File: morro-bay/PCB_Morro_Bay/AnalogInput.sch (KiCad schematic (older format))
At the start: 95 parts, among them SW1 SW_DIP_x10, SW2 SW_DIP_x10, U10 LM2902, U11 LM2902, U12 LM2902, U5 LM2902, U6 LM2902, U7 LM2902, U8 LM2902, U9 LM2902

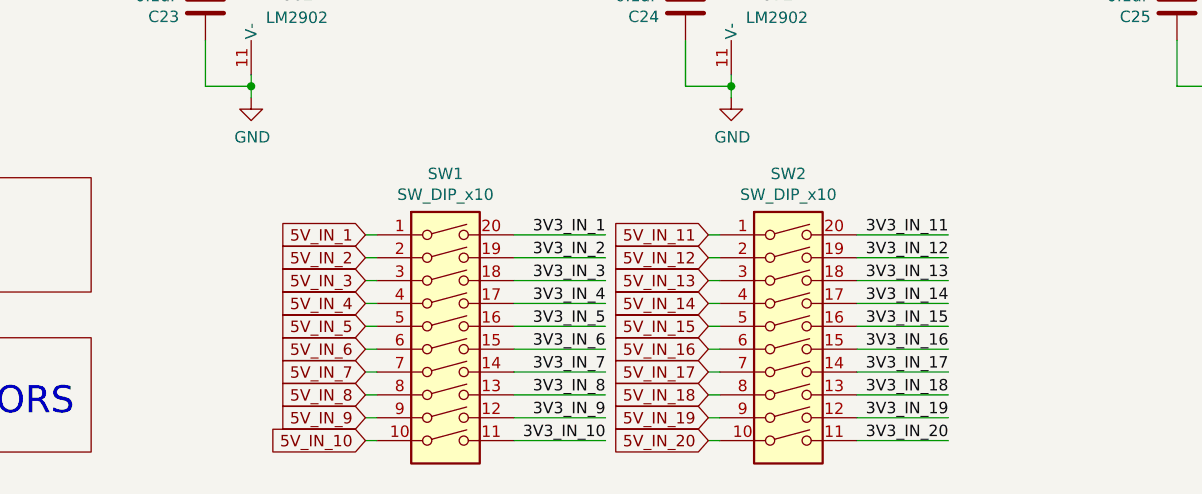
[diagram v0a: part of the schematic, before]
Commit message: Ready for initial sch review
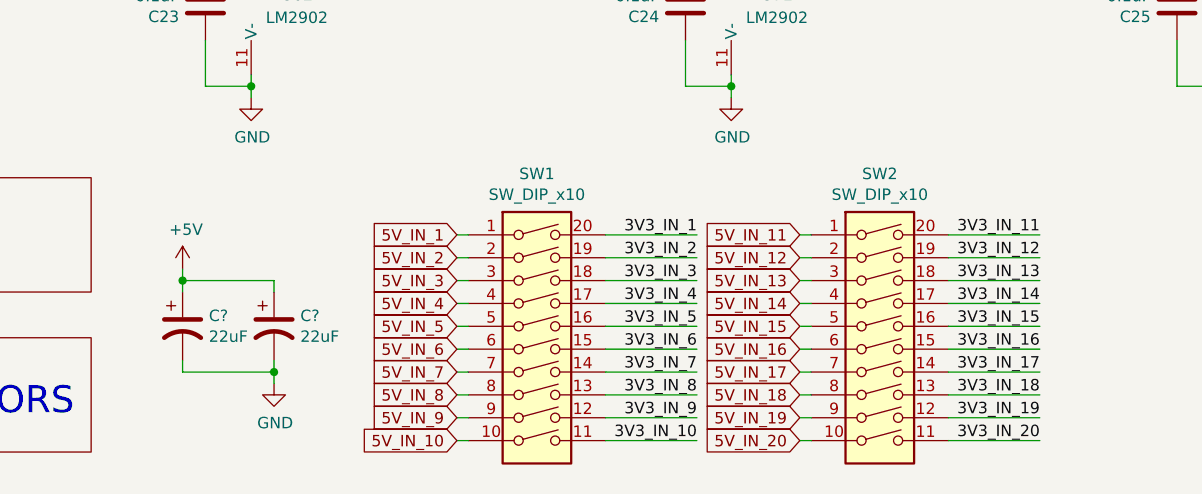
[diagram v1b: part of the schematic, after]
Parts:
- added C? (x2): 22uF, symbol Device:CP1
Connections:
- net +5V: now also C?.1, C?.1
- net GND: now also C?.2, C?.2
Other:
- moved on the sheet: SW1, SW2
